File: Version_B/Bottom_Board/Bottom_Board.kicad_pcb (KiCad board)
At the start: 2 copper layers, 74.8 x 84.5 mm, 47 parts, among them J1 Conn_02x03_Top_Bottom, J2 Conn_02x03_Top_Bottom, J3 Screw_Terminal_01x06, J5 DIN-5, SW2 SW_DIP_x04, U1 LM324, U2 LM324

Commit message: updated board b
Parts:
- C1, C8, C9: value .1uF -> 0.1uF
- C5: value .002uF -> 0.002uF
- C7: value 0.1 uF -> 0.1uF
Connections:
- J5 pad 6: AN1 -> (no net)
- J5 pad 7: AN1 -> (no net)
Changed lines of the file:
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@@
     (pad "5" thru_hole circle (at 5 8.5 270) (size 3 3) (drill 1.7) (layers "*.Cu" "*.Mask")
       (net 40 "12V") (pintype "passive"))
-    (pad "6" thru_hole circle (at -5 -3.5 270) (size 3 3) (drill 1.7) (layers "*.Cu" "*.Mask")
-      (net 3 "AN1"))
-    (pad "7" thru_hole circle (at 5 -3.5 270) (size 3 3) (drill 1.7) (layers "*.Cu" "*.Mask")
-      (net 3 "AN1"))
+    (pad "6" thru_hole circle (at -5 -3.5 270) (size 3 3) (drill 1.7) (layers "*.Cu" "*.Mask"))
+    (pad "7" thru_hole circle (at 5 -3.5 270) (size 3 3) (drill 1.7) (layers "*.Cu" "*.Mask"))
     (model "${KIPRJMOD}/Bottom_Board_3d/DIN_5_PIN.step"
       (offset (xyz 0 6.5 0))
@@
         (effects (font (size 1 1) (thickness 0.15)) (justify mirror))
     )
-    (fp_text value ".1uF" (at 1.425572 0.4125) (layer "B.Fab")
+    (fp_text value "0.1uF" (at 1.425572 0.4125) (layer "B.Fab")
         (effects (font (size 1 1) (thickness 0.15)) (justify mirror))
     )
@@
         (effects (font (size 1 1) (thickness 0.15)) (justify mirror))
     )
-    (fp_text value ".1uF" (at 0 -1.43) (layer "B.Fab")
+    (fp_text value "0.1uF" (at 0 -1.43) (layer "B.Fab")
         (effects (font (size 1 1) (thickness 0.15)) (justify mirror))
     )
@@
         (effects (font (size 1 1) (thickness 0.15)) (justify mirror))
     )
-    (fp_text value ".1uF" (at 1.956428 -4.064 90) (layer "B.Fab")
+    (fp_text value "0.1uF" (at 1.956428 -4.064 90) (layer "B.Fab")
         (effects (font (size 1 1) (thickness 0.15)) (justify mirror))
     )
@@
         (effects (font (size 1 1) (thickness 0.15)) (justify mirror))
     )
-    (fp_text value "0.1 uF" (at -0.0474 -1.3909) (layer "B.Fab")
+    (fp_text value "0.1uF" (at -0.0474 -1.3909) (layer "B.Fab")
         (effects (font (size 1 1) (thickness 0.15)) (justify mirror))
     )
@@
         (effects (font (size 1 1) (thickness 0.15)) (justify mirror))
     )
-    (fp_text value ".002uF" (at -4.060953 0) (layer "B.Fab")
+    (fp_text value "0.002uF" (at -4.060953 0) (layer "B.Fab")
         (effects (font (size 1 1) (thickness 0.15)) (justify mirror))
     )

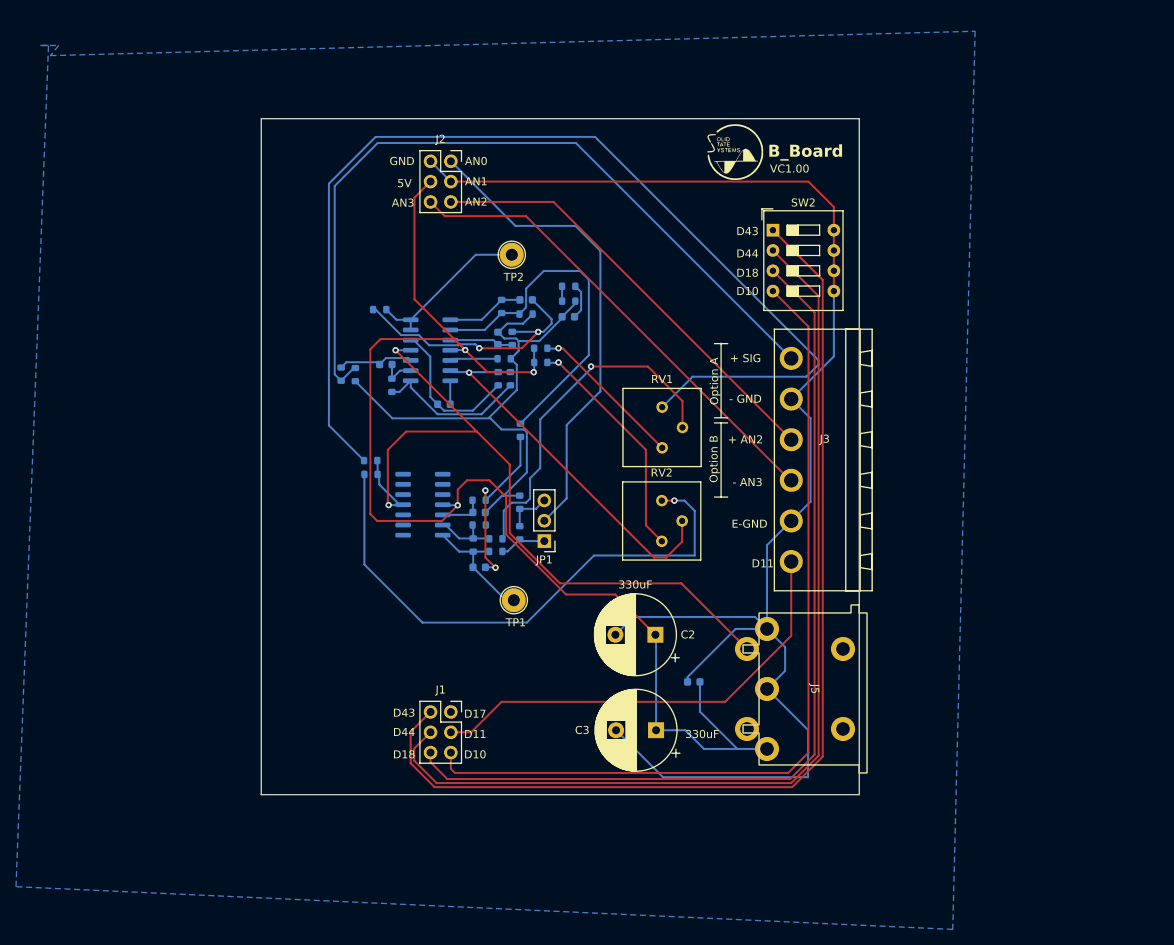
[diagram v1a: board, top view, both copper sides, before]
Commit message: updated simulation circuit and finalized hardware design?
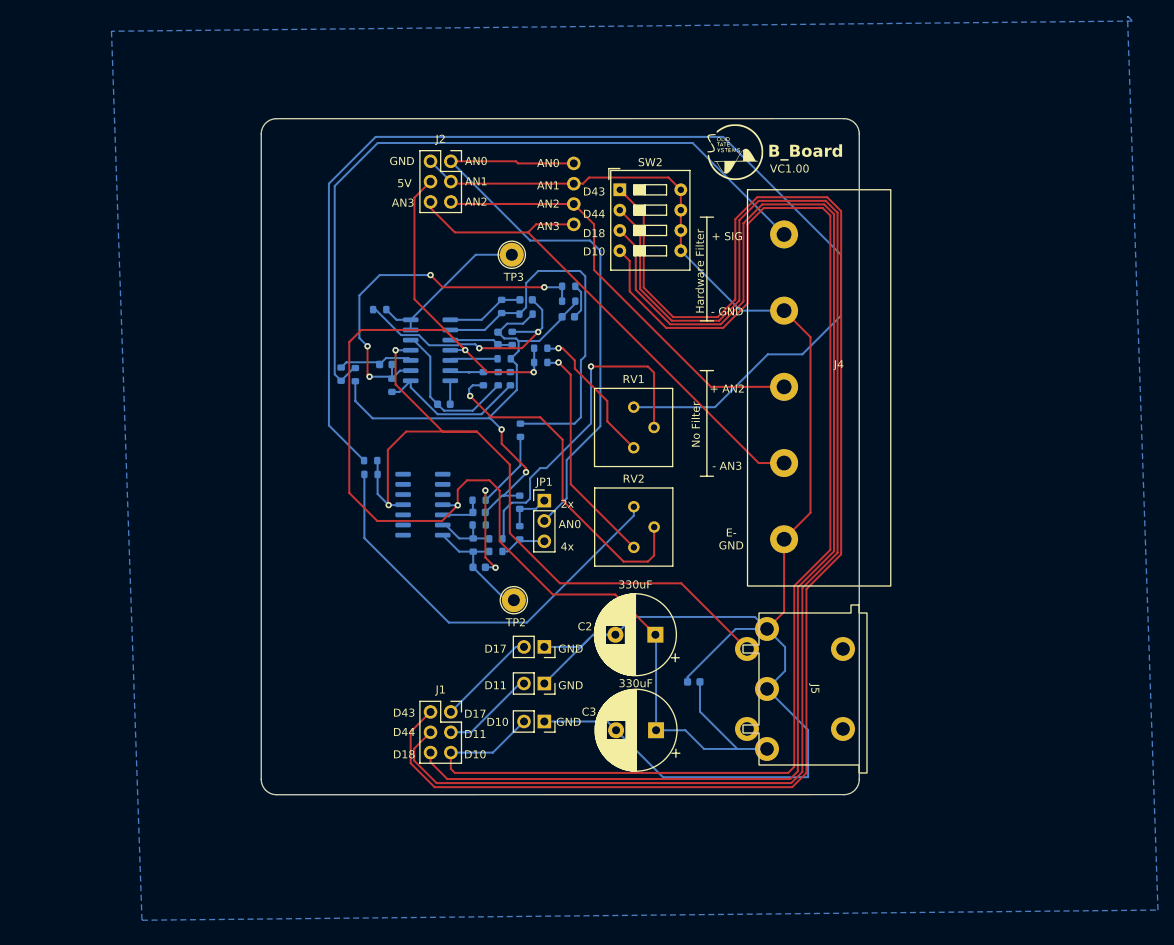
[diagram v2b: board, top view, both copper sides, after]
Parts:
- added J4: Screw_Terminal_01x05, bot_lib:BarrierStrip_1x05_P8.26mm_3.25in_Vertical, F.Cu at (165.4, 77.5)
- added J6: Conn_01x02_Pin, Connector_PinSocket_2.54mm:PinSocket_1x02_P2.54mm_Vertical, F.Cu at (135.4, 133.6)
- added J7: Conn_01x02_Pin, Connector_PinSocket_2.54mm:PinSocket_1x02_P2.54mm_Vertical, F.Cu at (135.4, 129.0)
- added J8: Screw_Terminal_01x04, Connector_PinHeader_2.54mm:PinHeader_1x04_P2.54mm_Vertical, F.Cu at (139.1, 68.6)
- added R25: 1M, Resistor_SMD:R_0603_1608Metric, B.Cu at (127.8, 95.5)
- J3: value Screw_Terminal_01x06 -> Conn_01x02_Pin; footprint Connector_Phoenix_MSTB:PhoenixContact_MSTBA_2,5_6-G-5,08_1x06_P5.08mm_Horizontal -> Connector_PinSocket_2.54mm:PinSocket_1x02_P2.54mm_Vertical
- moved J3 36.8 mm to (135.4, 138.4), turned to -90 degrees
- moved SW2 19.8 mm to (144.8, 71.9)
- moved JP1 5.05 mm to (135.4, 110.7), turned to 0 degrees
- moved RV2 3.58 mm to (146.6, 116.6)
- moved RV1 3.56 mm to (146.6, 104.1)
- renumbered TP1 to TP2, TP2 to TP3
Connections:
- J3 pad 1: D11 -> AN1
- J3 pad 2: AN1 -> D10
- R10 pad 1: Net-(R10-Pad1) -> Net-(U1C--)
- R12 pad 1: 2x_OUTPUT -> 4x_OUTPUT
- R13 pad 1: 4x_OUTPUT -> 2x_OUTPUT
- R13 pad 2: 2x_OUTPUT -> 4x_OUTPUT
- R14 pad 2: 4x_OUTPUT -> 2x_OUTPUT
- R7 pad 1: Net-(R10-Pad1) -> Net-(U1C--)
- RV2 pad 2: Net-(U1B--) -> Net-(R25-Pad2)
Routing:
- net D10: track 107.5 -> 172.0 mm
- net D44: track 123.0 -> 176.3 mm
- net D43: track 130.2 -> 183.4 mm
- net D18: track 114.0 -> 167.1 mm
- net D11: track 56.8 -> 11.7 mm
- net Net-(R25-Pad2): track 0.00 -> 42.8 mm, vias 0 -> 1
- net Net-(U1C--): track 4.56 -> 47.1 mm, vias 0 -> 4
- net Net-(U1B--): track 47.2 -> 7.64 mm, vias 1 -> 0
- net Net-(R18-Pad1): track 69.3 -> 52.7 mm, vias 1 -> 0
- net AN1: track 193.5 -> 209.5 mm
- net AN0: track 60.0 -> 75.4 mm
- net Net-(R3-Pad2): track 133.9 -> 147.2 mm
- net D17: track 0.00 -> 12.5 mm
- net E23_INPUT: track 97.6 -> 90.2 mm
- net 5V: track 161.7 -> 167.8 mm
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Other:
- outline, holes or cut-outs redrawn
- board text added: "2x"
- board text added: "4x"
- board text added: "E- GND"
- board text added: "No Filter"
- board text removed: "E-GND"
- board text removed: "Option A"
- board text removed: "Option B"
